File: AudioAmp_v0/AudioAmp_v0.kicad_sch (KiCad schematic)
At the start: 12 parts, among them J1 Conn_01x02_Pin, J2 AudioJack3, U1 MAU108, U2 NJM5532

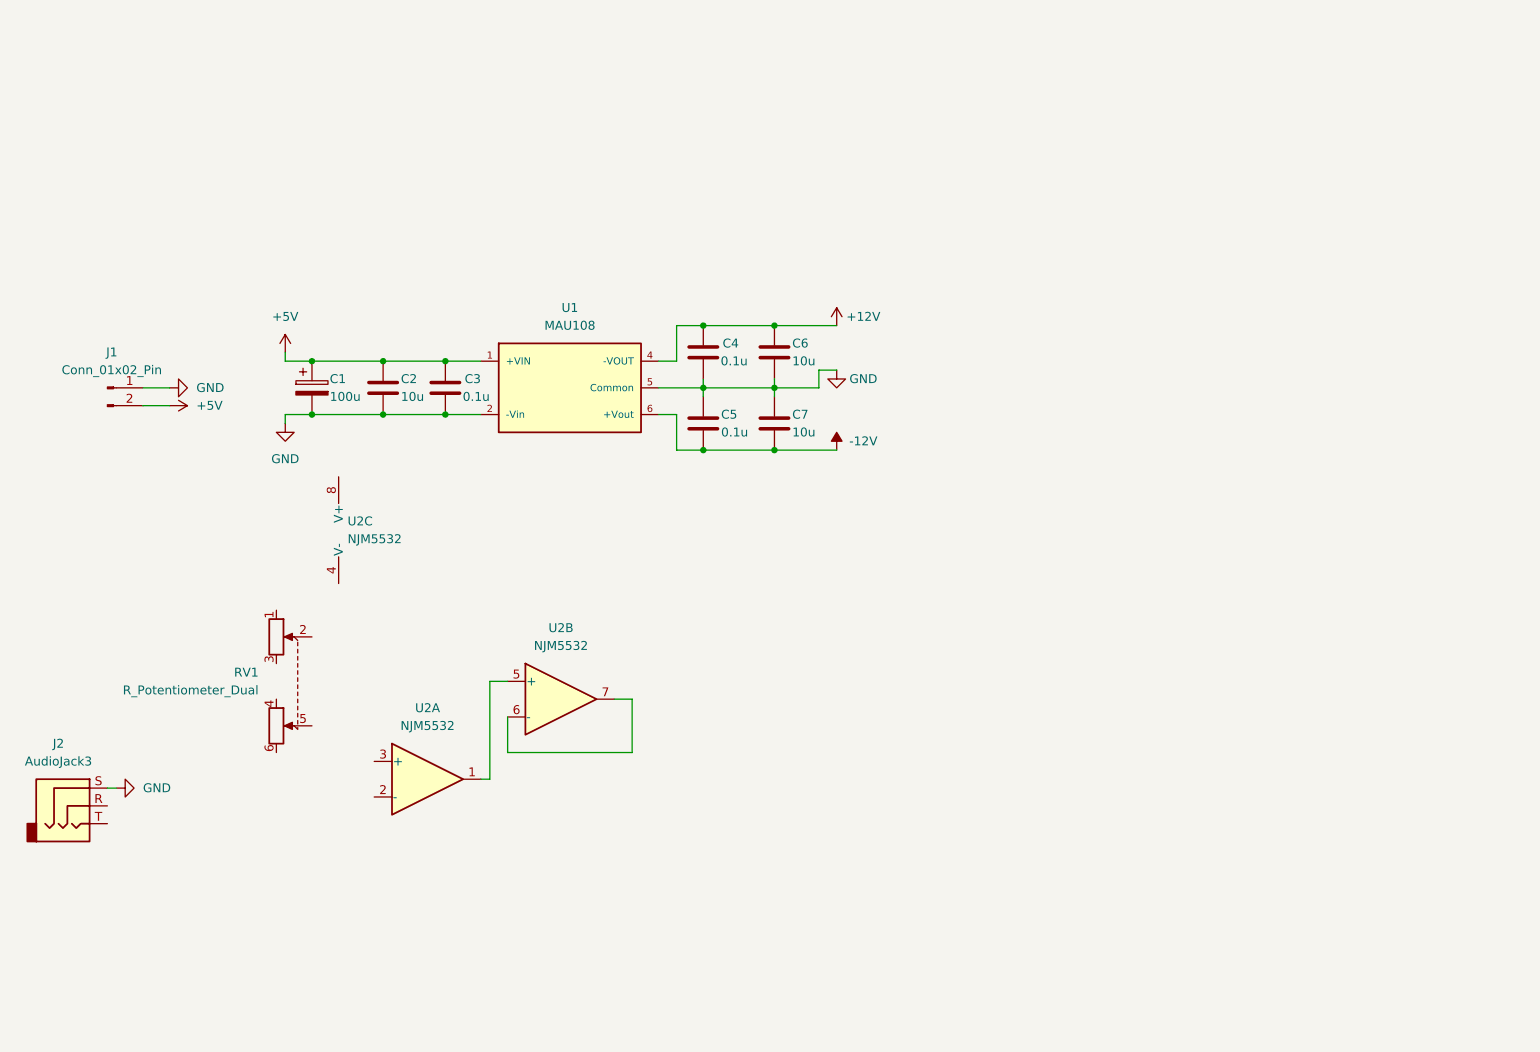
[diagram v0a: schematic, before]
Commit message: アンプ回路一応完成
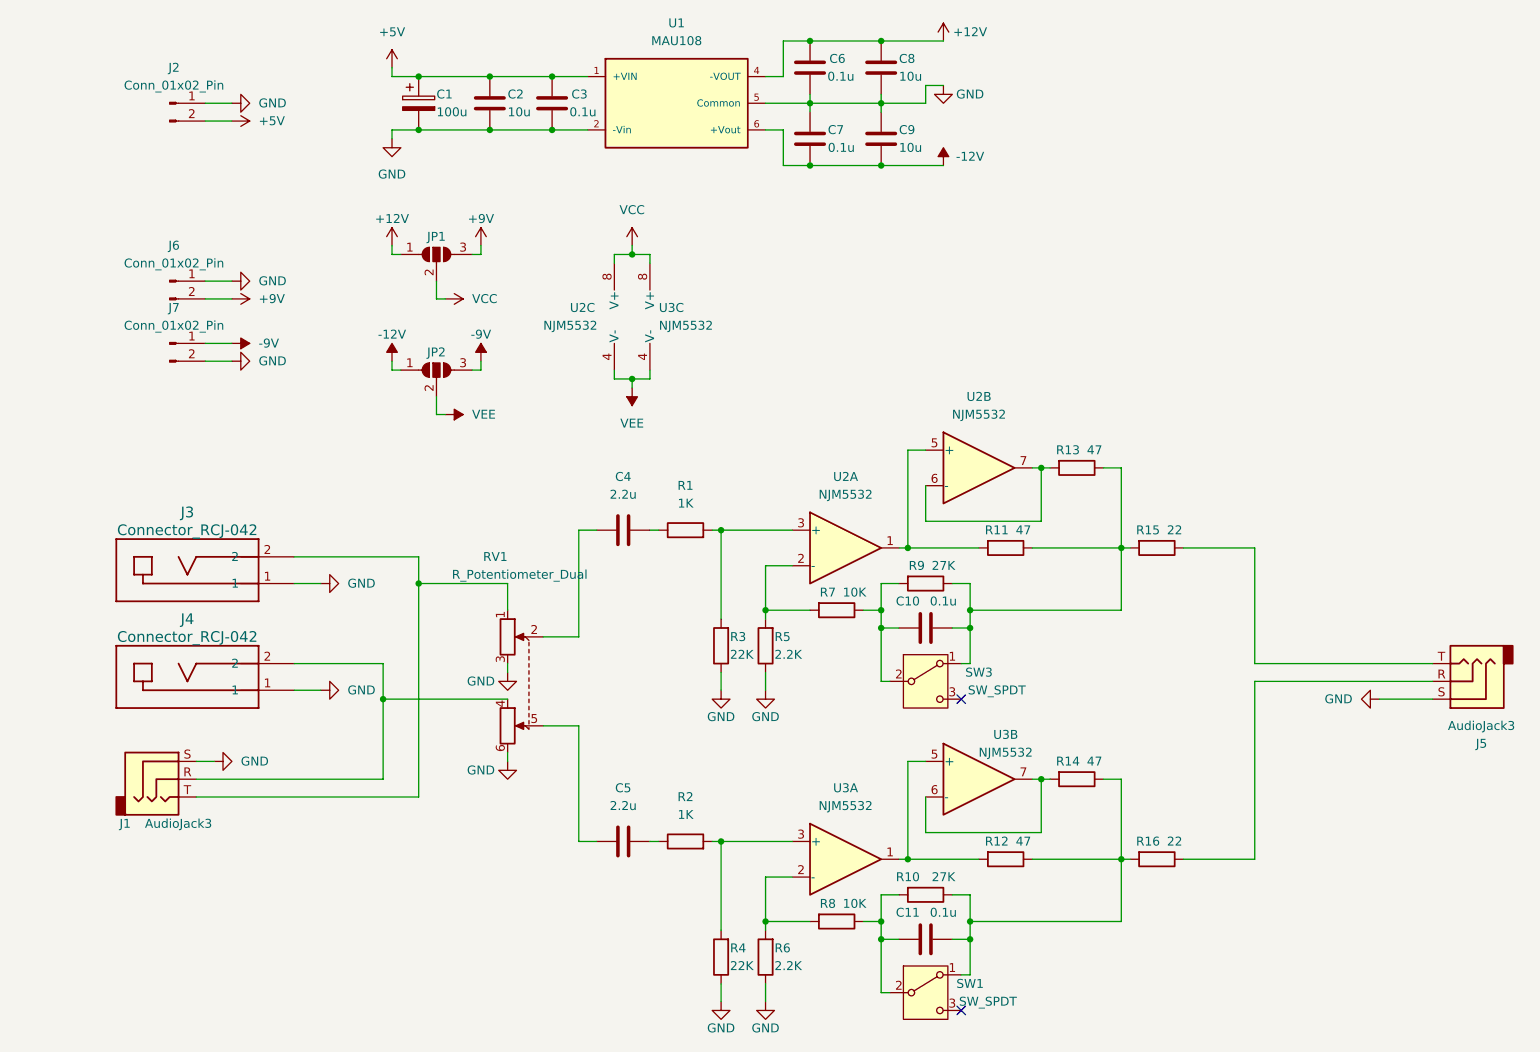
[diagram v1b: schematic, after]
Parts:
- added C10, C11: 0.1u, Capacitor_THT:C_Rect_L13.0mm_W6.0mm_P10.00mm_FKS3_FKP3_MKS4, symbol Device:C
- added C4, C5: 2.2u, Capacitor_THT:C_Axial_L17.0mm_D7.0mm_P20.00mm_Horizontal, symbol Device:C
- added J3, J4: Connector_RCJ-042, TomoshibiLibrary:Connector_RCJ-042CUD, symbol TomoshibiLibrary:Connector_RCJ-042
- added J5: AudioJack3, Connector_Audio:Jack_3.5mm_Switronic_ST-005-G_horizontal, symbol Connector_Audio:AudioJack3
- added J6, J7: Conn_01x02_Pin, Connector_JST:JST_XH_S2B-XH-A_1x02_P2.50mm_Horizontal, symbol Connector:Conn_01x02_Pin
- added JP1, JP2: SolderJumper_3_Open, Jumper:SolderJumper-3_P2.0mm_Open_TrianglePad1.0x1.5mm, symbol Jumper:SolderJumper_3_Open
- added R1, R2: 1K, Resistor_THT:R_Axial_DIN0207_L6.3mm_D2.5mm_P10.16mm_Horizontal, symbol Device:R
- added R10, R9: 27K, Resistor_THT:R_Axial_DIN0207_L6.3mm_D2.5mm_P10.16mm_Horizontal, symbol Device:R
- added R11, R12, R13, R14: 47, Resistor_THT:R_Axial_DIN0207_L6.3mm_D2.5mm_P10.16mm_Horizontal, symbol Device:R
- added R15, R16: 22, Resistor_THT:R_Axial_DIN0207_L6.3mm_D2.5mm_P10.16mm_Horizontal, symbol Device:R
- added R3, R4: 22K, Resistor_THT:R_Axial_DIN0207_L6.3mm_D2.5mm_P10.16mm_Horizontal, symbol Device:R
- added R5, R6: 2.2K, Resistor_THT:R_Axial_DIN0207_L6.3mm_D2.5mm_P10.16mm_Horizontal, symbol Device:R
- added R7, R8: 10K, Resistor_THT:R_Axial_DIN0207_L6.3mm_D2.5mm_P10.16mm_Horizontal, symbol Device:R
- added SW1, SW3: SW_SPDT, TomoshibiLibrary:SW_Toggle_3P_SPDT_5Pin, symbol Switch:SW_SPDT
- added U3: NJM5532, Package_DIP:DIP-8_W7.62mm, symbol Amplifier_Operational:NJM5532
- C1: footprint (none) -> Capacitor_SMD:CP_Elec_6.3x5.7
- RV1: footprint (none) -> TomoshibiLibrary:VR_ALPS9-dual
- renumbered C4 to C6, C5 to C7, C6 to C8, C7 to C9, J2 to J1, J1 to J2
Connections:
- net +12V: now also JP1.1 (A)
- net -12V: now also JP2.1 (A)
- net GND: now also RV1.3, RV1.6, J3.1, J4.1, J5.S, J6.1 (Pin_1), J7.2 (Pin_2), R3.1, R4.1, R5.1, R6.1
- net VEE: now reaches U2.4 (V-)
- net VEE: now also JP2.2 (C), U3.4 (V-)
- net VCC: now reaches U2.8 (V+)
- net VCC: now also JP1.2 (C), U3.8 (V+)
- net at J1.R: now also RV1.4, J4.2
- net at J1.T: now also RV1.1, J3.2
- net at RV1.2: now also C4.1
- net at RV1.5: now also C5.1
- net at U2.1, U2.5 (+): now also R11.2
- net at U2.2 (-): now also R5.2, R7.2
- net at U2.3 (+): now also R1.2, R3.2
- net at U2.6 (-), U2.7: now also R13.2
- new net: C5.2, R2.1
- new net: C4.2, R1.1
- new net: J5.T, R15.1
- new net: C10.2, R11.1, R13.1, R15.2, R9.1, SW3.1 (A)
- new net: C11.2, R10.1, R12.1, R14.1, R16.2, SW1.1 (A)
- new net: C11.1, R10.2, R8.1, SW1.2 (B)
- new net: J5.R, R16.1
- new net: R12.2, U3.1, U3.5 (+)
- new net: R14.2, U3.6 (-), U3.7
- new net: R6.2, R8.2, U3.2 (-)
- new net: C10.1, R7.1, R9.2, SW3.2 (B)
- new net: R2.2, R4.2, U3.3 (+)
- new net +9V: J6.2 (Pin_2), JP1.3 (B)
- new net -9V: J7.1 (Pin_1), JP2.3 (B)
- no-connect marks 0 -> 2
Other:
- moved on the sheet: C1, C2, C3, C6, C7, C8, C9, J1, J2, RV1, U1, U2A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
